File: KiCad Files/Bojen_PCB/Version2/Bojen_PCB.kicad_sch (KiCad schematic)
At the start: 28 parts, among them J1 5V Power In, J10 GPS EN, J11 Conn_02x08_Odd_Even, J12 Conn_02x08_Odd_Even, J13 Conn_02x08_Odd_Even, J14 Conn_02x08_Odd_Even, J15 Conn_02x08_Odd_Even, J16 Conn_02x08_Odd_Even, J17 Conn_02x08_Odd_Even, J18 Conn_02x08_Odd_Even, J19 Conn_02x08_Odd_Even, J2 Battery Voltage, J4 5V TFT, J5 3.3V TFT, J6 LED, J7 Conn_02x08_Odd_Even, J9 PWR TMR SKIP, U1 Display_TFT_1.8Zoll_ST7735, U13 Solar Controller, U2 NEO-GPS8M, U4 TLP5110 Power Timer Modul, U6 PCF8575 Module

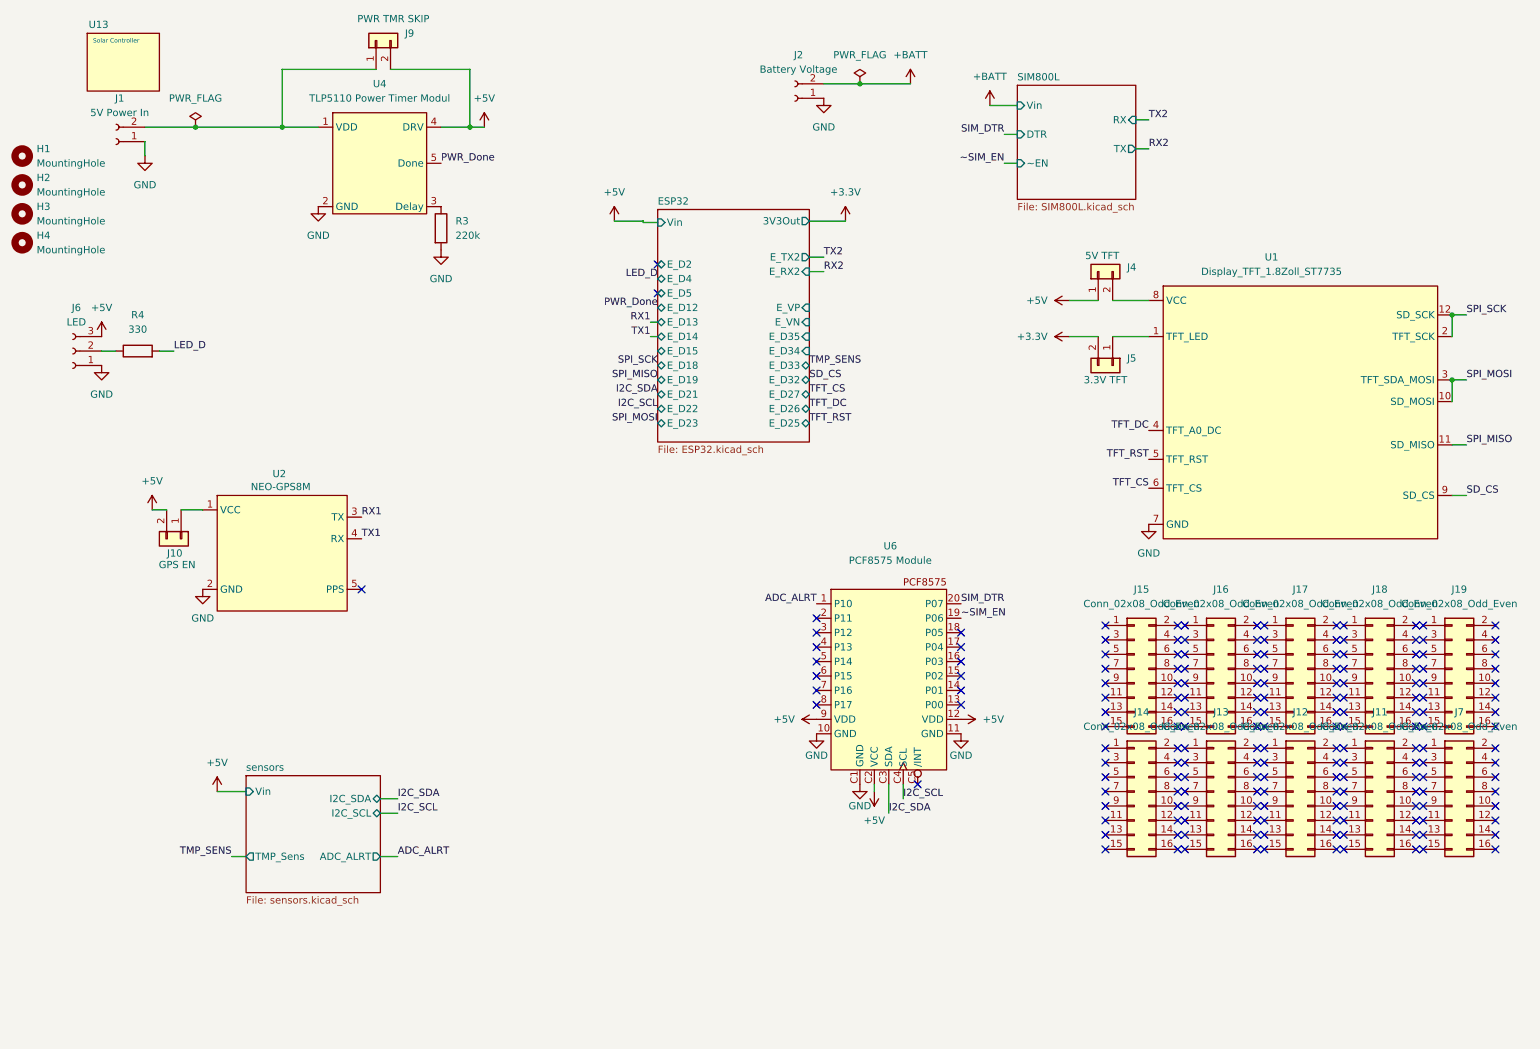
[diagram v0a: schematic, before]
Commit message: state_module, Bilder
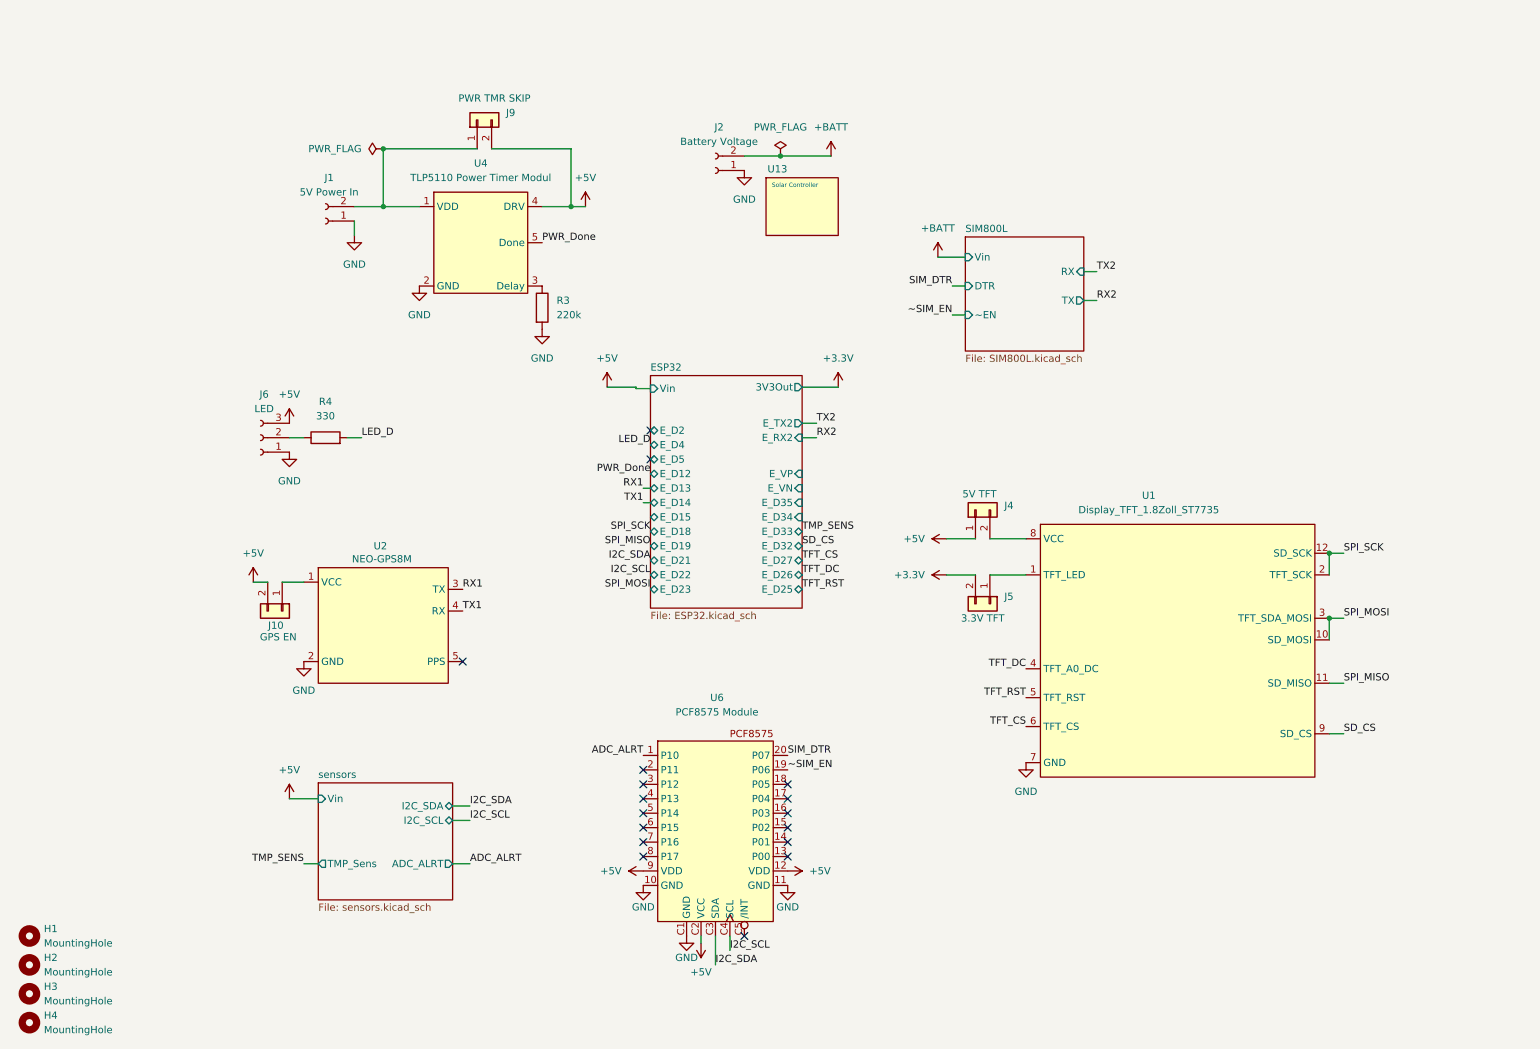
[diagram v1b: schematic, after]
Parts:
- removed J11, J12, J13, J14, J15, J16, J17, J18, J19, J7: Conn_02x08_Odd_Even, Connector_PinHeader_2.54mm:PinHeader_2x08_P2.54mm_Vertical, symbol Connector_Generic:Conn_02x08_Odd_Even
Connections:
- no-connect marks 177 -> 17
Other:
- company: (none) -> Alexander Mohr
- title: (none) -> Datenbojen
- moved on the sheet: H1, H2, H3, H4, J1, J10, J2, J4, J5, J6, J9, R3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
